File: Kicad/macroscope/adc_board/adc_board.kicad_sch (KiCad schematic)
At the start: 30 parts, among them J1 ADC board connector, J2 Bridge interface, U1 ADS1256IDBR, U2 AMS1117-3.3, U3 ADR4525, U4 OPA2356xxD, Y1 7.68MHz

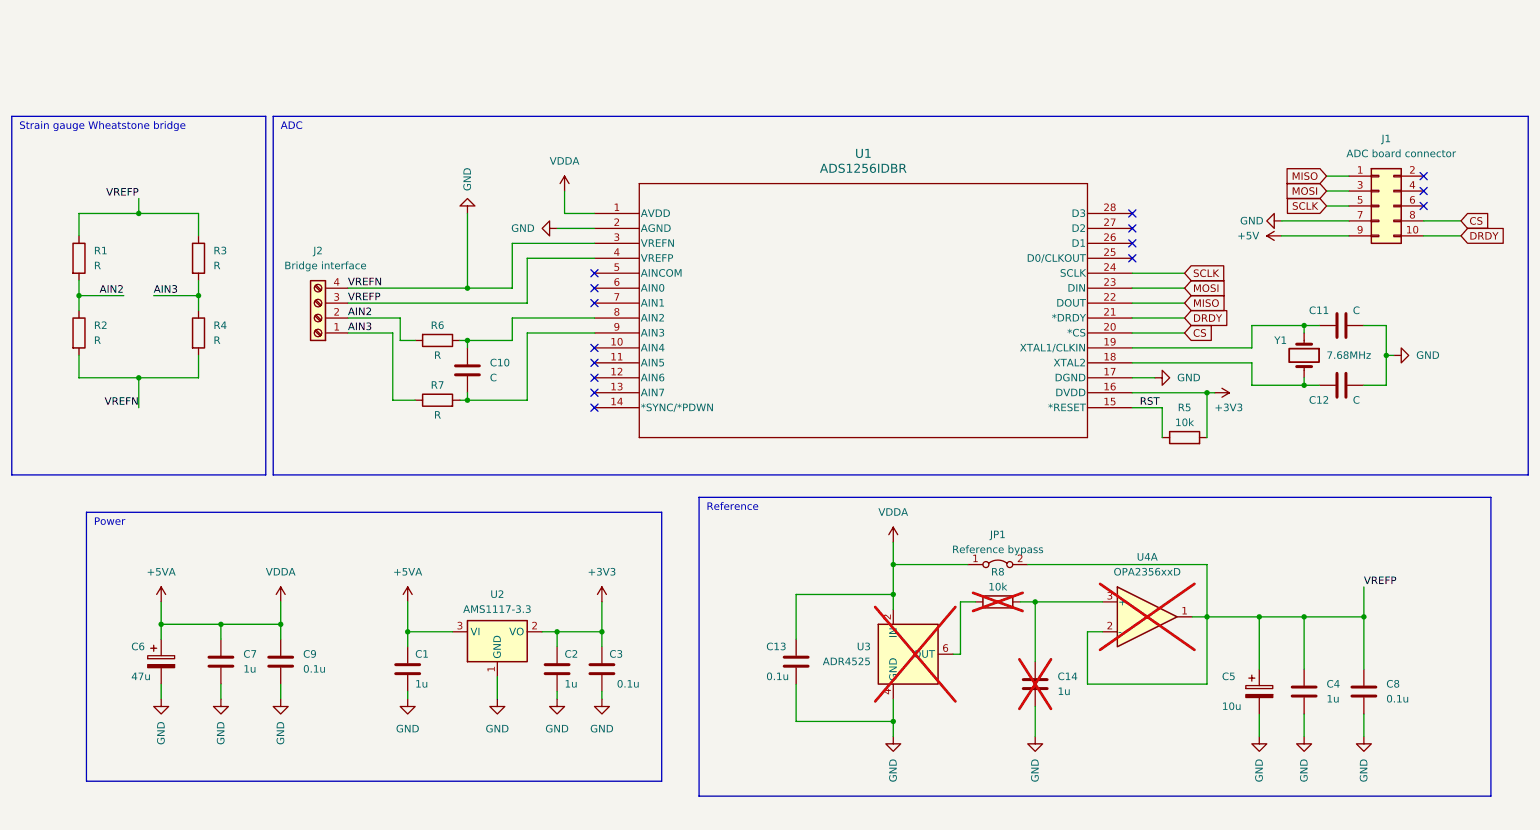
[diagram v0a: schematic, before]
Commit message: Update Kicad files
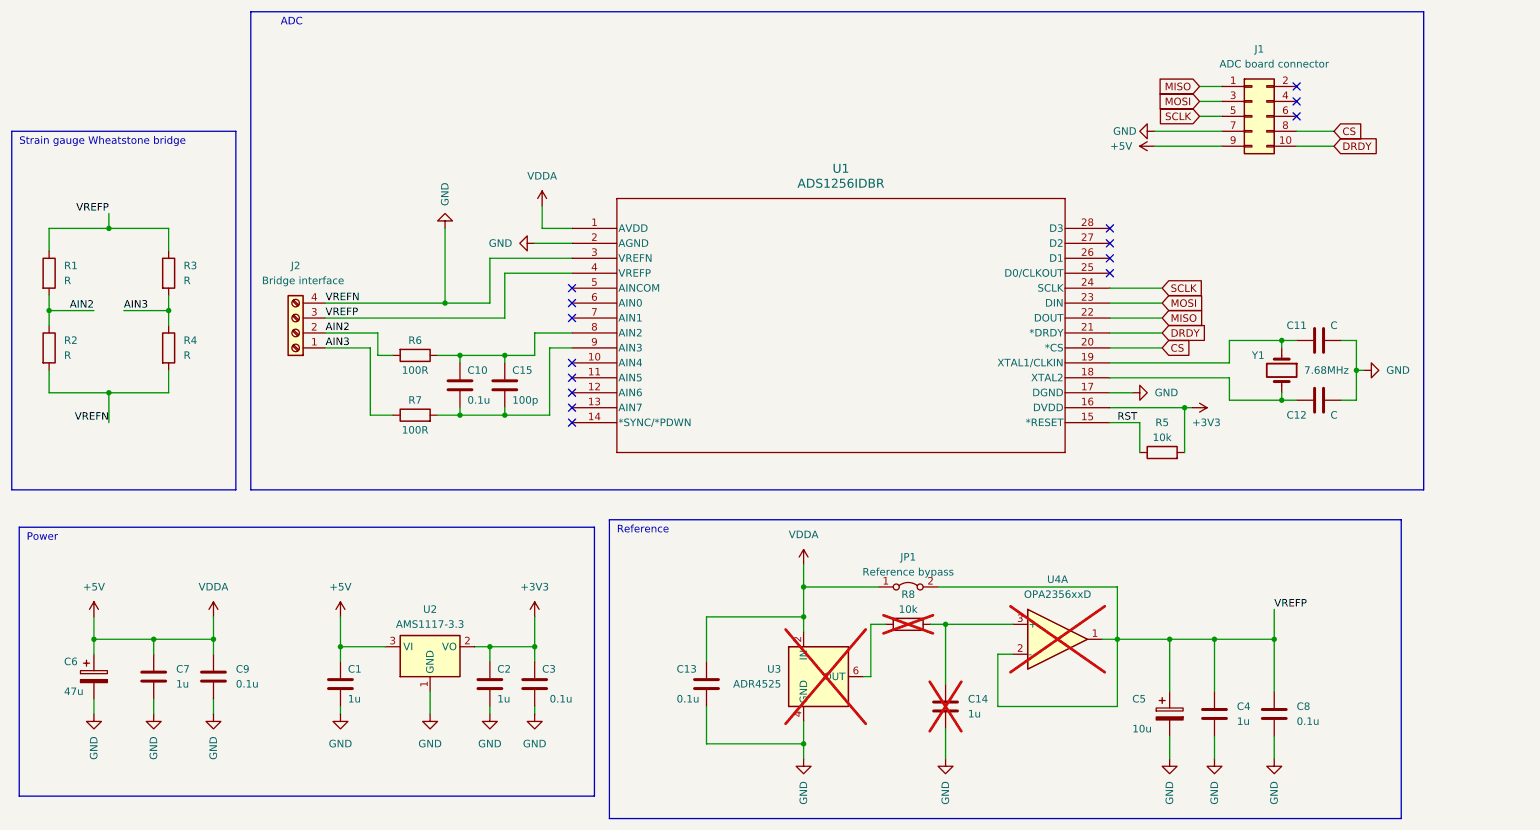
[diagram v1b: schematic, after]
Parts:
- added C15: 100p, symbol Device:C
- C10: value C -> 0.1u
- R6, R7: value R -> 100R
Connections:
- net +5VA is gone; now on net +5V: C1.1, C13.1, C6.1, C7.1, C9.1, JP1.1 (A), U1.1 (AVDD), U2.3 (VI), U3.2 (IN)
- net at C10.2, R7.2, U1.9 (AIN3): now also C15.2
- net at C10.1, R6.1, U1.8 (AIN2): now also C15.1
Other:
- moved on the sheet: C1, C10, C11, C12, C13, C14, C2, C3, C4, C5, C6, C7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

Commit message: Add CAD
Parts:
- U1: footprint DB28 -> Package_SO:SSOP-28_5.3x10.2mm_P0.65mm
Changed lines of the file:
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@@
       (effects (font (size 1.524 1.524)))
     )
-    (property "Footprint" "DB28" (at 115.57 62.23 0)
+    (property "Footprint" "Package_SO:SSOP-28_5.3x10.2mm_P0.65mm" (at 115.57 62.23 0)
       (effects (font (size 1.27 1.27) italic) hide)
     )
